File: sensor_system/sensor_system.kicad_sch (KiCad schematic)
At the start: 8 parts, among them U4 BME280, U5 ESP32-DEVKIT-V1

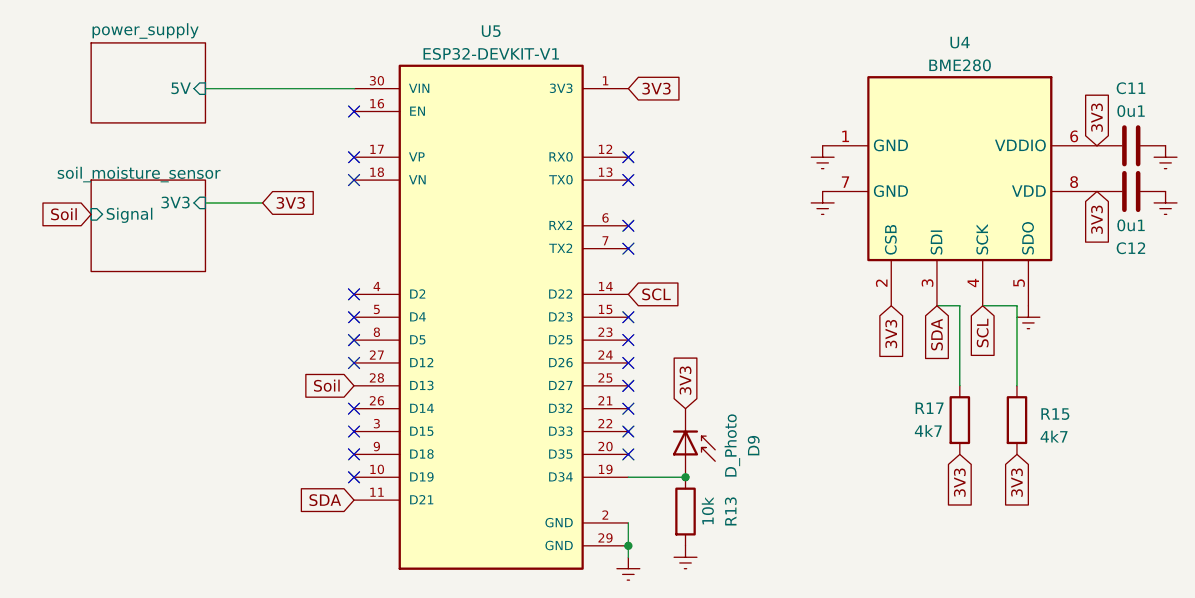
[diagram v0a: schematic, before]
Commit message: Board fix 2.0
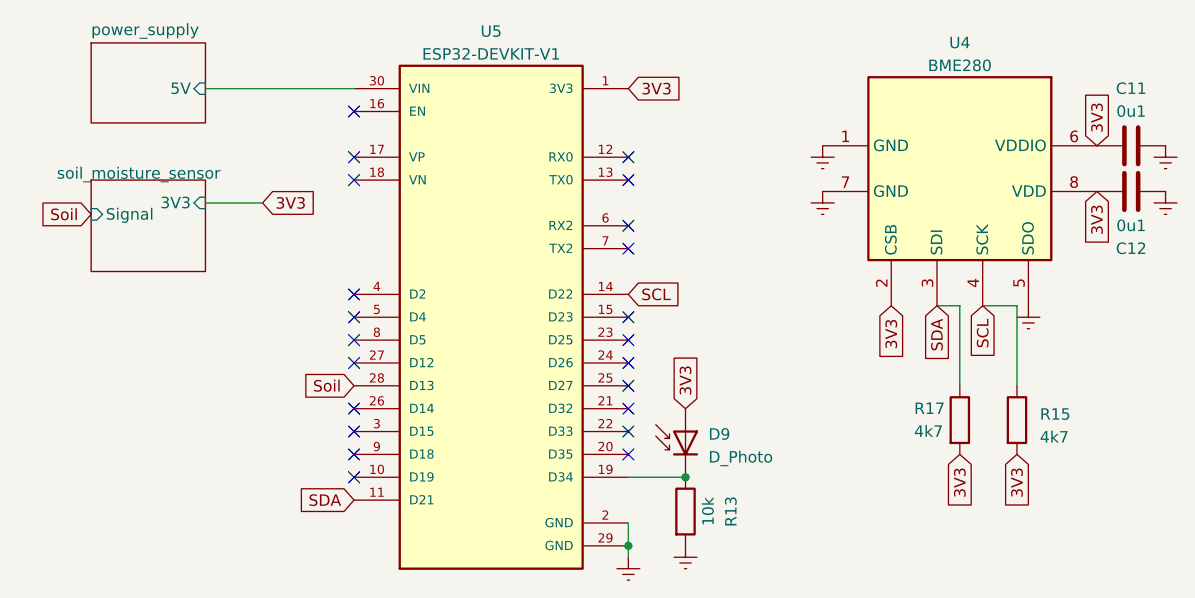
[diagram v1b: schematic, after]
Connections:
- net 3V3: now also D9.2 (A); no longer D9.1 (K)
- net at R13.1, U5.19 (D34): now also D9.1 (K); no longer D9.2 (A)
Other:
- moved on the sheet: D9
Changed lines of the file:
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@@
 (kicad_sch (version 20230121) (generator eeschema)
   (paper "A4")
+  (junction (at 102.87 81.28) (diameter 0) (color 0 0 0 0)
+  )
   (junction (at 109.22 73.66) (diameter 0) (color 0 0 0 0)
-  )
-  (junction (at 102.87 81.28) (diameter 0) (color 0 0 0 0)
   )
   (no_connect (at 72.39 60.96))
@@
     )
   )
-  (symbol (lib_id "Device:D_Photo") (at 109.22 71.12 270) (unit 1)
+  (symbol (lib_id "Device:D_Photo") (at 109.22 68.58 90) (unit 1)
     (in_bom yes) (on_board yes) (dnp no) (fields_autoplaced)
-    (property "Reference" "D9" (at 116.84 70.1675 0)
-      (effects (font (size 1.27 1.27)))
+    (property "Reference" "D9" (at 111.76 68.8975 90)
+      (effects (font (size 1.27 1.27)) (justify right))
     )
-    (property "Value" "D_Photo" (at 114.3 70.1675 0)
-      (effects (font (size 1.27 1.27)))
+    (property "Value" "D_Photo" (at 111.76 71.4375 90)
+      (effects (font (size 1.27 1.27)) (justify right))
     )
     (property "Footprint" "LED_THT:LED_D5.0mm" (at 109.22 69.85 0)
